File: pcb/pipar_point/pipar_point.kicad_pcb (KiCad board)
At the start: 2 copper layers, 32 parts, among them Y50 Crystal_GND2

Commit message: more pipar poimt progress
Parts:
- added AE1: Antenna, Mikoto:2.4GHz-meander-antenna-v2, B.Cu at (171.4, 61.8)
- added AE1: Antenna, Mikoto-Footprints:2.4GHz-meander-antenna-v2, B.Cu at (-137.7, 167.9)
- added AE2: Antenna, Mikoto:2.4GHz-meander-antenna-v2, B.Cu at (-153.7, 135.4)
- added C1: 4.7uF, Capacitor_SMD:C_0402_1005Metric, B.Cu at (-143.2, 159.1)
- added C1: 4.7uF, Capacitor_SMD:C_0402_1005Metric, B.Cu at (203.4, 69.8)
- added C10: 1.5pF, Capacitor_SMD:C_0402_1005Metric, B.Cu at (-144.8, 169.3)
- added C10: 1.5pF, Capacitor_SMD:C_0402_1005Metric, B.Cu at (198.5, 69.7)
- added C11: 1pF, Capacitor_SMD:C_0402_1005Metric, B.Cu at (196.9, 70.8)
- added C11: 1pF, Capacitor_SMD:C_0402_1005Metric, B.Cu at (-147.8, 168.9)
- added C12: 1pF, Capacitor_SMD:C_0402_1005Metric, B.Cu at (195.3, 71.9)
- added C12: 1pF, Capacitor_SMD:C_0402_1005Metric, B.Cu at (-149.9, 167.6)
- added C13: 4.7uF, Capacitor_SMD:C_0402_1005Metric, B.Cu at (193.7, 73.1)
- added C13: 4.7uF, Capacitor_SMD:C_0402_1005Metric, B.Cu at (-146.0, 157.0)
- added C14: 1uF, Capacitor_SMD:C_0402_1005Metric, B.Cu at (192.1, 74.2)
- added C14: 1uF, Capacitor_SMD:C_0402_1005Metric, B.Cu at (-135.2, 161.8)
- added C15: 1uF, Capacitor_SMD:C_0402_1005Metric, B.Cu at (-133.1, 164.8)
- added C15: 1uF, Capacitor_SMD:C_0402_1005Metric, B.Cu at (200.1, 65.1)
- added C16: 100nF, Capacitor_SMD:C_0402_1005Metric, B.Cu at (198.5, 66.2)
- added C16: 100nF, Capacitor_SMD:C_0402_1005Metric, B.Cu at (-155.1, 156.3)
- added C17: 100nF, Capacitor_SMD:C_0402_1005Metric, B.Cu at (196.9, 67.3)
- added C17: 100nF, Capacitor_SMD:C_0402_1005Metric, B.Cu at (-155.4, 164.1)
- added C18: 100nF, Capacitor_SMD:C_0402_1005Metric, B.Cu at (195.3, 68.4)
- added C18: 100nF, Capacitor_SMD:C_0402_1005Metric, B.Cu at (-141.6, 164.6)
- added C19: 4.7uF, Capacitor_SMD:C_0402_1005Metric, B.Cu at (193.7, 69.6)
- added C19: 4.7uF, Capacitor_SMD:C_0402_1005Metric, B.Cu at (-143.6, 156.5)
- added C2: 1uF, Capacitor_SMD:C_0402_1005Metric, B.Cu at (-151.8, 169.0)
- added C2: 1uF, Capacitor_SMD:C_0402_1005Metric, B.Cu at (201.8, 70.9)
- added C20: 1uF, Capacitor_SMD:C_0402_1005Metric, B.Cu at (192.1, 70.7)
- added C20: 1uF, Capacitor_SMD:C_0402_1005Metric, B.Cu at (-142.0, 162.5)
- added C21: 15pF, Capacitor_SMD:C_0402_1005Metric, B.Cu at (-155.2, 168.9)
- added C21: 15pF, Capacitor_SMD:C_0402_1005Metric, B.Cu at (190.4, 71.8)
- added C22: 15pF, Capacitor_SMD:C_0402_1005Metric, B.Cu at (-155.4, 165.1)
- added C22: 15pF, Capacitor_SMD:C_0402_1005Metric, B.Cu at (198.5, 62.7)
- added C23: 10nF, Capacitor_SMD:C_0402_1005Metric, B.Cu at (-136.2, 164.0)
- added C23: 10nF, Capacitor_SMD:C_0402_1005Metric, B.Cu at (196.9, 63.8)
- added C24: 1000pF/NC, Capacitor_SMD:C_0402_1005Metric, B.Cu at (195.2, 65.0)
- added C25: 1.5pF, Capacitor_SMD:C_0402_1005Metric, B.Cu at (-160.7, 136.8)
- added C26: 1pF, Capacitor_SMD:C_0402_1005Metric, B.Cu at (-164.3, 136.6)
- added C27: 15pF, Capacitor_SMD:C_0402_1005Metric, B.Cu at (-171.5, 137.2)
- added C28: 15pF, Capacitor_SMD:C_0402_1005Metric, B.Cu at (-171.9, 133.1)
- added C29: 1pF, Capacitor_SMD:C_0402_1005Metric, B.Cu at (-166.3, 134.9)
- added C3: 47nF, Capacitor_SMD:C_0402_1005Metric, B.Cu at (-154.2, 159.9)
- added C3: 47nF, Capacitor_SMD:C_0402_1005Metric, B.Cu at (200.2, 72.0)
- added C30: 100nF, Capacitor_SMD:C_0402_1005Metric, B.Cu at (-170.8, 124.3)
- added C31: 100pF, Capacitor_SMD:C_0402_1005Metric, B.Cu at (-169.1, 136.8)
- added C32: 1nF, Capacitor_SMD:C_0402_1005Metric, B.Cu at (-188.6, 182.0)
- added C33: 4.7uF, Capacitor_SMD:C_0402_1005Metric, B.Cu at (-159.5, 125.7)
- added C34: 4.7uF, Capacitor_SMD:C_0402_1005Metric, B.Cu at (-159.5, 126.7)
- added C35: 1uF, Capacitor_SMD:C_0402_1005Metric, B.Cu at (-168.1, 136.8)
- added C36: 47nF, Capacitor_SMD:C_0402_1005Metric, B.Cu at (-171.2, 128.3)
- added C37: 15pF, Capacitor_SMD:C_0402_1005Metric, B.Cu at (-168.8, 124.3)
- added C38: 15pF, Capacitor_SMD:C_0402_1005Metric, B.Cu at (-166.7, 122.9)
- added C39: 4.7uF, Capacitor_SMD:C_0402_1005Metric, B.Cu at (-162.5, 124.2)
- added C4: 4.7uF, Capacitor_SMD:C_0402_1005Metric, B.Cu at (198.6, 73.1)
- added C4: 4.7uF, Capacitor_SMD:C_0402_1005Metric, B.Cu at (-143.2, 158.1)
- added C40: 100nF, Capacitor_SMD:C_0402_1005Metric, B.Cu at (-171.8, 124.3)
- added C41: 10nF, Capacitor_SMD:C_0402_1005Metric, B.Cu at (-192.6, 179.1)
- added C42: 100nF, Capacitor_SMD:C_0402_1005Metric, B.Cu at (-158.4, 132.5)
- added C43: 100nF, Capacitor_SMD:C_0402_1005Metric, B.Cu at (-171.9, 132.1)
- added C44: 4.7uF, Capacitor_SMD:C_0402_1005Metric, B.Cu at (-160.3, 123.8)
- added C45: 1uF, Capacitor_SMD:C_0402_1005Metric, B.Cu at (-158.4, 130.1)
- added C46: 1000pF/NC, Capacitor_SMD:C_0402_1005Metric, B.Cu at (-188.6, 176.2)
- added C47: 1uF, Capacitor_SMD:C_0402_1005Metric, B.Cu at (-190.6, 176.2)
- added C48: 1uF, Capacitor_SMD:C_0402_1005Metric, B.Cu at (-192.6, 176.2)
- added C49: 10uF, Capacitor_SMD:C_0603_1608Metric, B.Cu at (191.6, 77.4)
- added C5: 1nF, Capacitor_SMD:C_0402_1005Metric, B.Cu at (-142.8, 166.5)
- added C5: 1nF, Capacitor_SMD:C_0402_1005Metric, B.Cu at (197.0, 74.3)
- added C6: 100pF, Capacitor_SMD:C_0402_1005Metric, B.Cu at (195.3, 75.4)
- added C6: 100pF, Capacitor_SMD:C_0402_1005Metric, B.Cu at (-152.8, 169.0)
- added C62: 4.7uF, Capacitor_SMD:C_0402_1005Metric, B.Cu at (193.6, 66.1)
- added C63: 10uF, Capacitor_SMD:C_0603_1608Metric, B.Cu at (-197.1, 180.9)
- added C64: 4.7uF, Capacitor_SMD:C_0402_1005Metric, B.Cu at (-194.5, 176.2)
- added C65: 100nF, Capacitor_SMD:C_0402_1005Metric, B.Cu at (192.0, 67.2)
- added C66: 100nF, Capacitor_SMD:C_0402_1005Metric, B.Cu at (-196.5, 176.2)
- added C7: 100nF, Capacitor_SMD:C_0402_1005Metric, B.Cu at (193.7, 76.5)
- added C7: 100nF, Capacitor_SMD:C_0402_1005Metric, B.Cu at (-154.0, 156.3)
- added C8: 15pF, Capacitor_SMD:C_0402_1005Metric, B.Cu at (201.8, 67.4)
- added C8: 15pF, Capacitor_SMD:C_0402_1005Metric, B.Cu at (-152.1, 156.8)
- added C9: 15pF, Capacitor_SMD:C_0402_1005Metric, B.Cu at (200.2, 68.5)
- added C9: 15pF, Capacitor_SMD:C_0402_1005Metric, B.Cu at (-150.1, 155.3)
- added D1: CHG, LED_SMD:LED_0603_1608Metric, B.Cu at (181.8, 79.3)
- added D100: D_Small, Diode_SMD:D_0402_1005Metric, B.Cu at (142.7, 121.5)
- added D101: D_Small, Diode_SMD:D_0402_1005Metric, B.Cu at (152.4, 135.4)
- added D102: D_Small, Diode_SMD:D_0402_1005Metric, B.Cu at (114.0, 114.5)
- added D103: D_Small, Diode_SMD:D_0402_1005Metric, B.Cu at (122.5, 129.2)
- added D104: D_Small, Diode_SMD:D_0402_1005Metric, B.Cu at (130.9, 143.9)
- added D105: D_Small, Diode_SMD:D_0402_1005Metric, B.Cu at (90.6, 111.2)
- added D106: D_Small, Diode_SMD:D_0402_1005Metric, B.Cu at (93.5, 127.9)
- added D107: D_Small, Diode_SMD:D_0402_1005Metric, B.Cu at (96.5, 144.6)
- added D108: D_Small, Diode_SMD:D_0402_1005Metric, B.Cu at (73.4, 118.9)
- added D109: D_Small, Diode_SMD:D_0402_1005Metric, B.Cu at (76.3, 135.6)
- added D110: D_Small, Diode_SMD:D_0402_1005Metric, B.Cu at (-138.0, 132.0)
- added D111: D_Small, Diode_SMD:D_0402_1005Metric, B.Cu at (-123.3, 142.3)
- added D112: D_Small, Diode_SMD:D_0402_1005Metric, B.Cu at (-108.6, 152.6)
- added D113: D_Small, Diode_SMD:D_0402_1005Metric, B.Cu at (-131.4, 76.9)
- added D114: D_Small, Diode_SMD:D_0402_1005Metric, B.Cu at (-132.9, 93.8)
- added D115: D_Small, Diode_SMD:D_0402_1005Metric, B.Cu at (-134.4, 110.7)
- added D116: D_Small, Diode_SMD:D_0402_1005Metric, B.Cu at (-150.1, 71.8)
- added D117: D_Small, Diode_SMD:D_0402_1005Metric, B.Cu at (-151.6, 88.7)
- added D118: D_Small, Diode_SMD:D_0402_1005Metric, B.Cu at (-153.1, 105.6)
- added D119: D_Small, Diode_SMD:D_0402_1005Metric, B.Cu at (-172.8, 70.0)
- added D120: D_Small, Diode_SMD:D_0402_1005Metric, B.Cu at (-172.8, 87.0)
- added D121: D_Small, Diode_SMD:D_0402_1005Metric, B.Cu at (-172.8, 104.0)
- added D122: D_Small, Diode_SMD:D_0402_1005Metric, B.Cu at (-195.2, 76.8)
- added D123: D_Small, Diode_SMD:D_0402_1005Metric, B.Cu at (-193.8, 93.7)
- added D124: D_Small, Diode_SMD:D_0402_1005Metric, B.Cu at (-192.3, 110.6)
- added D125: D_Small, Diode_SMD:D_0402_1005Metric, B.Cu at (-222.4, 101.6)
- added D126: D_Small, Diode_SMD:D_0402_1005Metric, B.Cu at (-215.2, 117.0)
- added D127: D_Small, Diode_SMD:D_0402_1005Metric, B.Cu at (-208.0, 132.3)
- added D128: D_Small, Diode_SMD:D_0402_1005Metric, B.Cu at (-233.8, 120.5)
- added D129: D_Small, Diode_SMD:D_0402_1005Metric, B.Cu at (-226.6, 135.9)
- added D2: B5819W SL, Diode_SMD:D_SOD-323, B.Cu at (186.0, 45.7)
- added D2: B5819W SL, Diode_SMD:D_SOD-323, B.Cu at (-130.2, 159.1)
- added D22: BLUE, LED_SMD:LED_0603_1608Metric, B.Cu at (177.5, 82.3)
- added D23: BLUE, LED_SMD:LED_0603_1608Metric, B.Cu at (-211.4, 176.8)
- added D3: BLUE, LED_SMD:LED_0603_1608Metric, B.Cu at (179.6, 80.8)
- added D4: BLUE, LED_SMD:LED_0603_1608Metric, B.Cu at (-206.3, 176.8)
- added D5: B5819W SL, Diode_SMD:D_SOD-323, B.Cu at (-186.4, 163.6)
- added D6: CHG, LED_SMD:LED_0603_1608Metric, B.Cu at (-208.8, 176.8)
- added D90: D_Small, Diode_SMD:D_0402_1005Metric, B.Cu at (149.7, 24.9)
- added D91: D_Small, Diode_SMD:D_0402_1005Metric, B.Cu at (143.6, 41.7)
- added D92: D_Small, Diode_SMD:D_0402_1005Metric, B.Cu at (137.5, 58.6)
- added D93: D_Small, Diode_SMD:D_0402_1005Metric, B.Cu at (181.5, 104.8)
- added D94: D_Small, Diode_SMD:D_0402_1005Metric, B.Cu at (170.6, 91.8)
- added D95: D_Small, Diode_SMD:D_0402_1005Metric, B.Cu at (159.7, 78.9)
- added D96: D_Small, Diode_SMD:D_0402_1005Metric, B.Cu at (147.3, 93.8)
- added D97: D_Small, Diode_SMD:D_0402_1005Metric, B.Cu at (158.2, 106.7)
- added D98: D_Small, Diode_SMD:D_0402_1005Metric, B.Cu at (169.1, 119.7)
- added D99: D_Small, Diode_SMD:D_0402_1005Metric, B.Cu at (133.0, 107.6)
- added H100: SwitchHoles, Keyboard:SwitchHoles_Kailh_Choc_V1V2, F.Cu at (135.9, 126.2)
- added H101: SwitchHoles, Keyboard:SwitchHoles_Kailh_Choc_V1V2, F.Cu at (145.6, 140.1)
- added H102: SwitchHoles, Keyboard:SwitchHoles_Kailh_Choc_V1V2, F.Cu at (106.8, 118.7)
- added H103: SwitchHoles, Keyboard:SwitchHoles_Kailh_Choc_V1V2, F.Cu at (115.3, 133.4)
- added H104: SwitchHoles, Keyboard:SwitchHoles_Kailh_Choc_V1V2, F.Cu at (123.8, 148.0)
- added H105: SwitchHoles, Keyboard:SwitchHoles_Kailh_Choc_V1V2, F.Cu at (82.4, 112.6)
- added H106: SwitchHoles, Keyboard:SwitchHoles_Kailh_Choc_V1V2, F.Cu at (85.4, 129.3)
- added H107: SwitchHoles, Keyboard:SwitchHoles_Kailh_Choc_V1V2, F.Cu at (88.3, 146.0)
- added H108: SwitchHoles, Keyboard:SwitchHoles_Kailh_Choc_V1V2, F.Cu at (65.2, 120.4)
- added H109: SwitchHoles, Keyboard:SwitchHoles_Kailh_Choc_V1V2, F.Cu at (68.1, 137.1)
- added H110: SwitchHoles, Keyboard:SwitchHoles_Kailh_Choc_V1V2, F.Cu at (-131.2, 136.7)
- added H111: SwitchHoles, Keyboard:SwitchHoles_Kailh_Choc_V1V2, F.Cu at (-116.5, 147.0)
- added H112: SwitchHoles, Keyboard:SwitchHoles_Kailh_Choc_V1V2, F.Cu at (-101.8, 157.3)
- added H113: SwitchHoles, Keyboard:SwitchHoles_Kailh_Choc_V1V2, F.Cu at (-123.1, 77.6)
- added H114: SwitchHoles, Keyboard:SwitchHoles_Kailh_Choc_V1V2, F.Cu at (-124.6, 94.5)
- added H115: SwitchHoles, Keyboard:SwitchHoles_Kailh_Choc_V1V2, F.Cu at (-126.1, 111.4)
- added H116: SwitchHoles, Keyboard:SwitchHoles_Kailh_Choc_V1V2, F.Cu at (-141.9, 72.6)
- added H117: SwitchHoles, Keyboard:SwitchHoles_Kailh_Choc_V1V2, F.Cu at (-143.3, 89.5)
- added H118: SwitchHoles, Keyboard:SwitchHoles_Kailh_Choc_V1V2, F.Cu at (-144.8, 106.3)
- added H119: SwitchHoles, Keyboard:SwitchHoles_Kailh_Choc_V1V2, F.Cu at (-164.5, 70.0)
- added H120: SwitchHoles, Keyboard:SwitchHoles_Kailh_Choc_V1V2, F.Cu at (-164.5, 87.0)
- added H121: SwitchHoles, Keyboard:SwitchHoles_Kailh_Choc_V1V2, F.Cu at (-164.5, 104.0)
- added H122: SwitchHoles, Keyboard:SwitchHoles_Kailh_Choc_V1V2, F.Cu at (-187.0, 76.1)
- added H123: SwitchHoles, Keyboard:SwitchHoles_Kailh_Choc_V1V2, F.Cu at (-185.5, 93.0)
- added H124: SwitchHoles, Keyboard:SwitchHoles_Kailh_Choc_V1V2, F.Cu at (-184.0, 109.9)
- added H125: SwitchHoles, Keyboard:SwitchHoles_Kailh_Choc_V1V2, F.Cu at (-214.8, 98.1)
- added H126: SwitchHoles, Keyboard:SwitchHoles_Kailh_Choc_V1V2, F.Cu at (-207.7, 113.5)
- added H127: SwitchHoles, Keyboard:SwitchHoles_Kailh_Choc_V1V2, F.Cu at (-200.5, 128.8)
- added H128: SwitchHoles, Keyboard:SwitchHoles_Kailh_Choc_V1V2, F.Cu at (-226.3, 117.0)
- added H129: SwitchHoles, Keyboard:SwitchHoles_Kailh_Choc_V1V2, F.Cu at (-219.1, 132.4)
- added H90: SwitchHoles, Keyboard:SwitchHoles_Kailh_Choc_V1V2, F.Cu at (146.9, 32.7)
- added H91: SwitchHoles, Keyboard:SwitchHoles_Kailh_Choc_V1V2, F.Cu at (140.8, 49.5)
- added H92: SwitchHoles, Keyboard:SwitchHoles_Kailh_Choc_V1V2, F.Cu at (134.6, 66.4)
- added H93: SwitchHoles, Keyboard:SwitchHoles_Kailh_Choc_V1V2, F.Cu at (175.2, 110.2)
- added H94: SwitchHoles, Keyboard:SwitchHoles_Kailh_Choc_V1V2, F.Cu at (164.3, 97.2)
- added H95: SwitchHoles, Keyboard:SwitchHoles_Kailh_Choc_V1V2, F.Cu at (153.4, 84.2)
- added H96: SwitchHoles, Keyboard:SwitchHoles_Kailh_Choc_V1V2, F.Cu at (141.0, 99.1)
- added H97: SwitchHoles, Keyboard:SwitchHoles_Kailh_Choc_V1V2, F.Cu at (151.8, 112.1)
- added H98: SwitchHoles, Keyboard:SwitchHoles_Kailh_Choc_V1V2, F.Cu at (162.7, 125.1)
- added H99: SwitchHoles, Keyboard:SwitchHoles_Kailh_Choc_V1V2, F.Cu at (126.2, 112.3)
- added J53: Conn_02x04_Odd_Even, Connector_PinHeader_2.54mm:PinHeader_2x04_P2.54mm_Vertical, F.Cu at (172.2, 46.2)
- added J54: Conn_02x04_Odd_Even, Connector_PinHeader_2.54mm:PinHeader_2x04_P2.54mm_Vertical_SMD, B.Cu at (-228.4, 104.7)
- added KHS100: KHS, Keyboard:Kailh_HS_Socket, F.Cu at (135.2, 120.8)
- added KHS101: KHS, Keyboard:Kailh_HS_Socket, F.Cu at (144.9, 134.7)
- added KHS102: KHS, Keyboard:Kailh_HS_Socket, F.Cu at (106.5, 113.2)
- added KHS103: KHS, Keyboard:Kailh_HS_Socket, F.Cu at (115.0, 127.9)
- added KHS104: KHS, Keyboard:Kailh_HS_Socket, F.Cu at (123.5, 142.5)
- added KHS105: KHS, Keyboard:Kailh_HS_Socket, F.Cu at (84.1, 107.4)
- added KHS106: KHS, Keyboard:Kailh_HS_Socket, F.Cu at (87.0, 124.1)
- added KHS107: KHS, Keyboard:Kailh_HS_Socket, F.Cu at (89.9, 140.8)
- added KHS108: KHS, Keyboard:Kailh_HS_Socket, F.Cu at (66.8, 115.1)
- added KHS109: KHS, Keyboard:Kailh_HS_Socket, F.Cu at (69.8, 131.8)
- added KHS110: KHS, Keyboard:Kailh_HS_Socket, F.Cu at (-136.1, 139.3)
- added KHS111: KHS, Keyboard:Kailh_HS_Socket, F.Cu at (-121.4, 149.6)
- added KHS112: KHS, Keyboard:Kailh_HS_Socket, F.Cu at (-106.7, 159.9)
- added KHS113: KHS, Keyboard:Kailh_HS_Socket, F.Cu at (-126.1, 82.3)
- added KHS114: KHS, Keyboard:Kailh_HS_Socket, F.Cu at (-127.5, 99.2)
- added KHS115: KHS, Keyboard:Kailh_HS_Socket, F.Cu at (-129.0, 116.1)
- added KHS116: KHS, Keyboard:Kailh_HS_Socket, F.Cu at (-144.8, 77.2)
- added KHS117: KHS, Keyboard:Kailh_HS_Socket, F.Cu at (-146.3, 94.1)
- added KHS118: KHS, Keyboard:Kailh_HS_Socket, F.Cu at (-147.7, 111.0)
- added KHS119: KHS, Keyboard:Kailh_HS_Socket, F.Cu at (-167.0, 74.9)
- added KHS120: KHS, Keyboard:Kailh_HS_Socket, F.Cu at (-167.0, 91.9)
- added KHS121: KHS, Keyboard:Kailh_HS_Socket, F.Cu at (-167.0, 108.9)
- added KHS122: KHS, Keyboard:Kailh_HS_Socket, F.Cu at (-189.1, 81.2)
- added KHS123: KHS, Keyboard:Kailh_HS_Socket, F.Cu at (-187.6, 98.1)
- added KHS124: KHS, Keyboard:Kailh_HS_Socket, F.Cu at (-186.1, 115.0)
- added KHS125: KHS, Keyboard:Kailh_HS_Socket, F.Cu at (-215.0, 103.6)
- added KHS126: KHS, Keyboard:Kailh_HS_Socket, F.Cu at (-207.9, 119.0)
- added KHS127: KHS, Keyboard:Kailh_HS_Socket, F.Cu at (-200.7, 134.3)
- added KHS128: KHS, Keyboard:Kailh_HS_Socket, F.Cu at (-226.5, 122.5)
- added KHS129: KHS, Keyboard:Kailh_HS_Socket, F.Cu at (-219.3, 137.9)
- added KHS90: KHS, Keyboard:Kailh_HS_Socket, F.Cu at (143.2, 28.6)
- added KHS91: KHS, Keyboard:Kailh_HS_Socket, F.Cu at (137.0, 45.5)
- added KHS92: KHS, Keyboard:Kailh_HS_Socket, F.Cu at (130.9, 62.4)
- added KHS93: KHS, Keyboard:Kailh_HS_Socket, F.Cu at (174.0, 104.8)
- added KHS94: KHS, Keyboard:Kailh_HS_Socket, F.Cu at (163.0, 91.8)
- added KHS95: KHS, Keyboard:Kailh_HS_Socket, F.Cu at (152.2, 78.8)
- added KHS96: KHS, Keyboard:Kailh_HS_Socket, F.Cu at (139.7, 93.7)
- added KHS97: KHS, Keyboard:Kailh_HS_Socket, F.Cu at (150.6, 106.7)
- added KHS98: KHS, Keyboard:Kailh_HS_Socket, F.Cu at (161.5, 119.7)
- added KHS99: KHS, Keyboard:Kailh_HS_Socket, F.Cu at (125.4, 106.9)
- added L1: 15nH, Inductor_SMD:L_0402_1005Metric, B.Cu at (171.2, 66.9)
- added L1: 15nH, Inductor_SMD:L_0402_1005Metric, B.Cu at (-157.3, 159.9)
- added L2: 10uH, Inductor_SMD:L_0603_1608Metric, B.Cu at (189.5, 78.8)
- added L2: 10uH, Inductor_SMD:L_0603_1608Metric, B.Cu at (-156.7, 158.6)
- added L3: 10uH, Inductor_SMD:L_0603_1608Metric, B.Cu at (-145.7, 155.7)
- added L3: 10uH, Inductor_SMD:L_0603_1608Metric, B.Cu at (187.5, 80.2)
- added L4: 3.9nH, Inductor_SMD:L_0402_1005Metric, B.Cu at (-147.8, 167.9)
- added L4: 3.9nH, Inductor_SMD:L_0402_1005Metric, B.Cu at (169.6, 68.1)
- added L5: 3.9nH, Inductor_SMD:L_0402_1005Metric, B.Cu at (-164.3, 135.6)
- added L6: 15nH, Inductor_SMD:L_0402_1005Metric, B.Cu at (-173.7, 127.8)
- added L7: 10uH, Inductor_SMD:L_0603_1608Metric, B.Cu at (-173.2, 126.5)
- added L8: 10uH, Inductor_SMD:L_0603_1608Metric, B.Cu at (-162.5, 122.9)
- added LED100: LED_Small, LED_SMD:LED_0402_1005Metric, F.Cu at (139.0, 130.5)
- added LED101: LED_Small, LED_SMD:LED_0402_1005Metric, F.Cu at (148.7, 144.4)
- added LED102: LED_Small, LED_SMD:LED_0402_1005Metric, F.Cu at (109.4, 123.2)
- added LED103: LED_Small, LED_SMD:LED_0402_1005Metric, F.Cu at (117.9, 137.9)
- added LED104: LED_Small, LED_SMD:LED_0402_1005Metric, F.Cu at (126.4, 152.6)
- added LED105: LED_Small, LED_SMD:LED_0402_1005Metric, F.Cu at (83.4, 117.8)
- added LED106: LED_Small, LED_SMD:LED_0402_1005Metric, F.Cu at (86.3, 134.5)
- added LED107: LED_Small, LED_SMD:LED_0402_1005Metric, F.Cu at (89.3, 151.2)
- added LED108: LED_Small, LED_SMD:LED_0402_1005Metric, F.Cu at (66.1, 125.5)
- added LED109: LED_Small, LED_SMD:LED_0402_1005Metric, F.Cu at (69.1, 142.3)
- added LED110: LED_Small, LED_SMD:LED_0402_1005Metric, F.Cu at (-128.2, 132.5)
- added LED111: LED_Small, LED_SMD:LED_0402_1005Metric, F.Cu at (-113.5, 142.8)
- added LED112: LED_Small, LED_SMD:LED_0402_1005Metric, F.Cu at (-98.7, 153.1)
- added LED113: LED_Small, LED_SMD:LED_0402_1005Metric, F.Cu at (-122.6, 72.5)
- added LED114: LED_Small, LED_SMD:LED_0402_1005Metric, F.Cu at (-124.1, 89.4)
- added LED115: LED_Small, LED_SMD:LED_0402_1005Metric, F.Cu at (-125.5, 106.3)
- added LED116: LED_Small, LED_SMD:LED_0402_1005Metric, F.Cu at (-141.3, 67.4)
- added LED117: LED_Small, LED_SMD:LED_0402_1005Metric, F.Cu at (-142.8, 84.3)
- added LED118: LED_Small, LED_SMD:LED_0402_1005Metric, F.Cu at (-144.3, 101.2)
- added LED119: LED_Small, LED_SMD:LED_0402_1005Metric, F.Cu at (-164.4, 64.8)
- added LED120: LED_Small, LED_SMD:LED_0402_1005Metric, F.Cu at (-164.4, 81.8)
- added LED121: LED_Small, LED_SMD:LED_0402_1005Metric, F.Cu at (-164.4, 98.7)
- added LED122: LED_Small, LED_SMD:LED_0402_1005Metric, F.Cu at (-187.3, 70.9)
- added LED123: LED_Small, LED_SMD:LED_0402_1005Metric, F.Cu at (-185.9, 87.8)
- added LED124: LED_Small, LED_SMD:LED_0402_1005Metric, F.Cu at (-184.4, 104.7)
- added LED125: LED_Small, LED_SMD:LED_0402_1005Metric, F.Cu at (-217.0, 93.3)
- added LED126: LED_Small, LED_SMD:LED_0402_1005Metric, F.Cu at (-209.8, 108.7)
- added LED127: LED_Small, LED_SMD:LED_0402_1005Metric, F.Cu at (-202.6, 124.1)
- added LED128: LED_Small, LED_SMD:LED_0402_1005Metric, F.Cu at (-228.4, 112.2)
- added LED129: LED_Small, LED_SMD:LED_0402_1005Metric, F.Cu at (-221.2, 127.6)
- added LED90: LED_Small, LED_SMD:LED_0402_1005Metric, F.Cu at (151.8, 34.6)
- added LED91: LED_Small, LED_SMD:LED_0402_1005Metric, F.Cu at (145.7, 51.4)
- added LED92: LED_Small, LED_SMD:LED_0402_1005Metric, F.Cu at (139.5, 68.3)
- added LED93: LED_Small, LED_SMD:LED_0402_1005Metric, F.Cu at (178.5, 114.3)
- added LED94: LED_Small, LED_SMD:LED_0402_1005Metric, F.Cu at (167.6, 101.2)
- added LED95: LED_Small, LED_SMD:LED_0402_1005Metric, F.Cu at (156.8, 88.2)
- added LED96: LED_Small, LED_SMD:LED_0402_1005Metric, F.Cu at (144.4, 103.1)
- added LED97: LED_Small, LED_SMD:LED_0402_1005Metric, F.Cu at (155.1, 116.2)
- added LED98: LED_Small, LED_SMD:LED_0402_1005Metric, F.Cu at (166.1, 129.1)
- added LED99: LED_Small, LED_SMD:LED_0402_1005Metric, F.Cu at (129.2, 116.6)
- added LR100: R_Small, Resistor_SMD:R_0402_1005Metric, F.Cu at (138.4, 129.7)
- added LR101: R_Small, Resistor_SMD:R_0402_1005Metric, F.Cu at (148.1, 143.6)
- added LR102: R_Small, Resistor_SMD:R_0402_1005Metric, F.Cu at (108.9, 122.3)
- added LR103: R_Small, Resistor_SMD:R_0402_1005Metric, F.Cu at (117.4, 137.0)
- added LR104: R_Small, Resistor_SMD:R_0402_1005Metric, F.Cu at (125.9, 151.7)
- added LR105: R_Small, Resistor_SMD:R_0402_1005Metric, F.Cu at (83.2, 116.8)
- added LR106: R_Small, Resistor_SMD:R_0402_1005Metric, F.Cu at (86.1, 133.5)
- added LR107: R_Small, Resistor_SMD:R_0402_1005Metric, F.Cu at (89.1, 150.2)
- added LR108: R_Small, Resistor_SMD:R_0402_1005Metric, F.Cu at (65.9, 124.6)
- added LR109: R_Small, Resistor_SMD:R_0402_1005Metric, F.Cu at (68.9, 141.3)
- added LR110: R_Small, Resistor_SMD:R_0402_1005Metric, F.Cu at (-128.7, 133.3)
- added LR111: R_Small, Resistor_SMD:R_0402_1005Metric, F.Cu at (-114.0, 143.6)
- added LR112: R_Small, Resistor_SMD:R_0402_1005Metric, F.Cu at (-99.3, 153.9)
- added LR113: R_Small, Resistor_SMD:R_0402_1005Metric, F.Cu at (-122.7, 73.5)
- added LR114: R_Small, Resistor_SMD:R_0402_1005Metric, F.Cu at (-124.2, 90.4)
- added LR115: R_Small, Resistor_SMD:R_0402_1005Metric, F.Cu at (-125.6, 107.3)
- added LR116: R_Small, Resistor_SMD:R_0402_1005Metric, F.Cu at (-141.4, 68.4)
- added LR117: R_Small, Resistor_SMD:R_0402_1005Metric, F.Cu at (-142.9, 85.3)
- added LR118: R_Small, Resistor_SMD:R_0402_1005Metric, F.Cu at (-144.4, 102.2)
- added LR119: R_Small, Resistor_SMD:R_0402_1005Metric, F.Cu at (-164.4, 65.8)
- added LR120: R_Small, Resistor_SMD:R_0402_1005Metric, F.Cu at (-164.4, 82.8)
- added LR121: R_Small, Resistor_SMD:R_0402_1005Metric, F.Cu at (-164.4, 99.7)
- added LR122: R_Small, Resistor_SMD:R_0402_1005Metric, F.Cu at (-187.2, 71.9)
- added LR123: R_Small, Resistor_SMD:R_0402_1005Metric, F.Cu at (-185.8, 88.8)
- added LR124: R_Small, Resistor_SMD:R_0402_1005Metric, F.Cu at (-184.3, 105.7)
- added LR125: R_Small, Resistor_SMD:R_0402_1005Metric, F.Cu at (-216.5, 94.2)
- added LR126: R_Small, Resistor_SMD:R_0402_1005Metric, F.Cu at (-209.4, 109.6)
- added LR127: R_Small, Resistor_SMD:R_0402_1005Metric, F.Cu at (-202.2, 125.0)
- added LR128: R_Small, Resistor_SMD:R_0402_1005Metric, F.Cu at (-227.9, 113.1)
- added LR129: R_Small, Resistor_SMD:R_0402_1005Metric, F.Cu at (-220.8, 128.5)
- added LR90: R_Small, Resistor_SMD:R_0402_1005Metric, F.Cu at (150.9, 34.2)
- added LR91: R_Small, Resistor_SMD:R_0402_1005Metric, F.Cu at (144.7, 51.1)
- added LR92: R_Small, Resistor_SMD:R_0402_1005Metric, F.Cu at (138.6, 68.0)
- added LR93: R_Small, Resistor_SMD:R_0402_1005Metric, F.Cu at (177.8, 113.5)
- added LR94: R_Small, Resistor_SMD:R_0402_1005Metric, F.Cu at (167.0, 100.4)
- added LR95: R_Small, Resistor_SMD:R_0402_1005Metric, F.Cu at (156.1, 87.4)
- added LR96: R_Small, Resistor_SMD:R_0402_1005Metric, F.Cu at (143.7, 102.3)
- added LR97: R_Small, Resistor_SMD:R_0402_1005Metric, F.Cu at (154.5, 115.4)
- added LR98: R_Small, Resistor_SMD:R_0402_1005Metric, F.Cu at (165.5, 128.3)
- added LR99: R_Small, Resistor_SMD:R_0402_1005Metric, F.Cu at (128.6, 115.8)
- added NT1: NetTie_2, Mikoto-Footprints:net-tie-2-tiny, B.Cu at (-150.2, 164.8)
- added NT1: NetTie_2, Mikoto:net-tie-2-tiny, B.Cu at (161.5, 61.1)
- added NT2: NetTie_2, Mikoto:net-tie-2-tiny, B.Cu at (-166.5, 132.4)
- added P1: USB-C, Connector_USB:USB_C_Receptacle_HRO_TYPE-C-31-M-12, B.Cu at (190.4, 59.5)
- added P2: USB-C, Connector_USB:USB_C_Receptacle_HRO_TYPE-C-31-M-12, B.Cu at (-121.2, 125.8)
- added Q1: AO3416 N-channel MOSFET, Package_TO_SOT_SMD:SOT-23, B.Cu at (181.8, 49.1)
- added Q2: AO3416 N-channel MOSFET, Package_TO_SOT_SMD:SOT-23, B.Cu at (-191.8, 164.0)
- added R1: 0R, Resistor_SMD:R_0402_1005Metric, B.Cu at (167.9, 69.2)
- added R1: 0R, Resistor_SMD:R_0402_1005Metric, B.Cu at (-144.8, 167.8)
- added R10: 10M, Resistor_SMD:R_0402_1005Metric, B.Cu at (-136.2, 165.0)
- added R10: 10M, Resistor_SMD:R_0402_1005Metric, B.Cu at (167.9, 62.1)
- added R11: 1M, Resistor_SMD:R_0402_1005Metric, B.Cu at (166.2, 63.3)
- added R12: 0R, Resistor_SMD:R_0402_1005Metric, B.Cu at (-160.7, 135.6)
- added R13: 2M, Resistor_SMD:R_0603_1608Metric, B.Cu at (-204.6, 180.9)
- added R14: 2M, Resistor_SMD:R_0603_1608Metric, B.Cu at (-207.2, 180.9)
- added R15: 10M, Resistor_SMD:R_0402_1005Metric, B.Cu at (-216.6, 172.5)
- added R16: 1.5k, Resistor_SMD:R_0402_1005Metric, B.Cu at (-210.6, 169.6)
- added R17: 1M, Resistor_SMD:R_0402_1005Metric, B.Cu at (-212.6, 169.6)
- added R18: 2.7k, Resistor_SMD:R_0603_1608Metric, B.Cu at (-209.7, 180.9)
- added R19: 10k, Resistor_SMD:R_0402_1005Metric, B.Cu at (-214.6, 169.6)
- added R2: 10k, Resistor_SMD:R_0402_1005Metric, B.Cu at (166.3, 70.3)
- added R2: 10k, Resistor_SMD:R_0402_1005Metric, B.Cu at (-134.6, 159.6)
- added R20: 5.1k, Resistor_SMD:R_0402_1005Metric, B.Cu at (-216.6, 169.6)
- added R21: 5.1k, Resistor_SMD:R_0402_1005Metric, B.Cu at (-210.6, 166.7)
- added R22: 10k, Resistor_SMD:R_0402_1005Metric, B.Cu at (-212.6, 166.7)
- added R23: 2M, Resistor_SMD:R_0402_1005Metric, B.Cu at (164.6, 64.4)
- added R24: 2M, Resistor_SMD:R_0402_1005Metric, B.Cu at (-214.6, 166.7)
- added R3: 2.7k, Resistor_SMD:R_0603_1608Metric, B.Cu at (185.4, 81.7)
- added R3: 2.7k, Resistor_SMD:R_0603_1608Metric, B.Cu at (-130.1, 162.6)
- added R31: 1.5k, Resistor_SMD:R_0402_1005Metric, B.Cu at (163.0, 65.6)
- added R32: 1.5k, Resistor_SMD:R_0402_1005Metric, B.Cu at (-216.6, 166.7)
- added R39: 4.7k, Resistor_SMD:R_0402_1005Metric_Pad0.72x0.64mm_HandSolder, B.Cu at (163.8, 61.3)
- added R4: 10k, Resistor_SMD:R_0402_1005Metric, B.Cu at (169.5, 64.5)
- added R4: 10k, Resistor_SMD:R_0402_1005Metric, B.Cu at (-135.2, 162.9)
- added R40: 4.7k, Resistor_SMD:R_0402_1005Metric_Pad0.72x0.64mm_HandSolder, B.Cu at (-213.5, 163.6)
- added R5: 1.5k, Resistor_SMD:R_0402_1005Metric, B.Cu at (167.9, 65.7)
- added R6: 5.1k, Resistor_SMD:R_0402_1005Metric, B.Cu at (166.3, 66.8)
- added R7: 5.1k, Resistor_SMD:R_0402_1005Metric, B.Cu at (164.6, 68.0)
- added R8: 2M, Resistor_SMD:R_0603_1608Metric, B.Cu at (183.3, 83.1)
- added R8: 2M, Resistor_SMD:R_0603_1608Metric, B.Cu at (-135.9, 159.7)
- added R9: 2M, Resistor_SMD:R_0603_1608Metric, B.Cu at (181.3, 84.6)
- added R9: 2M, Resistor_SMD:R_0603_1608Metric, B.Cu at (-137.5, 161.0)
- added SW1: Reset, Keyboard:SW4-SMD-2.8-2.6X1.6X0.53MM, B.Cu at (174.7, 72.4)
- added SW2: Reset, Keyboard:SW4-SMD-2.8-2.6X1.6X0.53MM, B.Cu at (-208.1, 167.2)
- added TP5: VBAT, TestPoint:TestPoint_Pad_2.5x2.5mm, B.Cu at (188.3, 74.4)
- added TP6: BAT GND, TestPoint:TestPoint_Pad_2.5x2.5mm, B.Cu at (184.6, 77.0)
- added TP7: VBAT, TestPoint:TestPoint_Pad_2.5x2.5mm, B.Cu at (-197.9, 166.9)
- added TP8: BAT GND, TestPoint:TestPoint_Pad_2.5x2.5mm, B.Cu at (-202.4, 166.9)
- added U1: BQ21040DBVR, BQ21040:SOT95P280X145-6N, B.Cu at (-132.5, 161.7)
- added U1: BQ21040DBVR, Mikoto:SOT95P280X145-6N, B.Cu at (188.1, 50.0)
- added U10: MAX17048, Package_DFN_QFN:TDFN-8-1EP_2x2mm_P0.5mm_EP0.8x1.2mm, B.Cu at (-216.2, 180.2)
- added U2: nRF52840, Package_DFN_QFN:Nordic_AQFN-73-1EP_7x7mm_P0.5mm, B.Cu at (-148.7, 162.3)
- added U2: nRF52840, Package_DFN_QFN:Nordic_AQFN-73-1EP_7x7mm_P0.5mm, B.Cu at (177.5, 58.1)
- added U3: ESDR0502NMUTAG, Mikoto:UDFN-6_1.2x1.0mm_P0.4mm, B.Cu at (162.3, 62.9)
- added U4: nRF52840, Package_DFN_QFN:Nordic_AQFN-73-1EP_7x7mm_P0.5mm, B.Cu at (-165.0, 129.8)
- added U5: ESDR0502NMUTAG, Mikoto:UDFN-6_1.2x1.0mm_P0.4mm, B.Cu at (-215.7, 164.1)
- added U6: BQ21040DBVR, Mikoto:SOT95P280X145-6N, B.Cu at (-187.1, 168.4)
- added U7: XC6220B331MR, Package_TO_SOT_SMD:SOT-23-5, B.Cu at (184.7, 53.2)
- added U8: XC6220B331MR, Package_TO_SOT_SMD:SOT-23-5, B.Cu at (-191.8, 169.0)
- added U9: MAX17048, Package_DFN_QFN:TDFN-8-1EP_2x2mm_P0.5mm_EP0.8x1.2mm, B.Cu at (171.5, 76.9)
- added Y1: 32.768 kHz, Crystal:Crystal_SMD_2012-2Pin_2.0x1.2mm, B.Cu at (-150.2, 156.8)
- added Y1: 32.768 kHz, Crystal:Crystal_SMD_2012-2Pin_2.0x1.2mm, B.Cu at (165.6, 59.7)
- added Y2: 32MHz, Crystal:Crystal_SMD_2016-4Pin_2.0x1.6mm, B.Cu at (-155.0, 167.0)
- added Y2: 32MHz, Crystal:Crystal_SMD_2016-4Pin_2.0x1.6mm, B.Cu at (169.2, 73.6)
- added Y3: 32MHz, Crystal:Crystal_SMD_2016-4Pin_2.0x1.6mm, B.Cu at (-171.5, 135.4)
- added Y4: 32.768 kHz, Crystal:Crystal_SMD_2012-2Pin_2.0x1.2mm, B.Cu at (-166.9, 124.3)
- C50, C51, C52, C53, C54, C55, C56, C57, C58, C59, C60, C61, R50, R51, R52, R53, R54, R55, R56, R57, R58, R59, R60, R61, R62, R63, R64, R65, U50, U51, Y50: moved to B.Cu
- moved C50 65.6 mm to (212.7, 111.3), turned to 125 degrees
- moved C51 64.0 mm to (213.2, 108.5), turned to -145 degrees
- moved C52 60.4 mm to (212.1, 106.7), turned to -55 degrees
- moved R50 58.5 mm to (210.8, 107.1), turned to 125 degrees
- moved R51 57.5 mm to (209.9, 107.7), turned to 125 degrees
- moved R52 56.4 mm to (210.7, 105.0), turned to 35 degrees
- moved R55 54.5 mm to (210.1, 104.1), turned to 35 degrees
- moved U50 54.2 mm to (206.3, 111.0), turned to -145 degrees
- moved R54 53.7 mm to (208.9, 105.5), turned to -55 degrees
- moved R56 52.7 mm to (209.5, 103.2), turned to 35 degrees
- moved C55 50.9 mm to (208.9, 102.3), turned to -145 degrees
- moved R57 50.4 mm to (207.8, 103.9), turned to -55 degrees
- moved C59 48.2 mm to (208.2, 100.7), turned to 125 degrees
- moved C60 47.1 mm to (207.1, 101.4), turned to 125 degrees
- moved C53 40.4 mm to (200.6, 106.4), turned to 125 degrees
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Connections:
- R60 pad 1: /Trackpointer/Vcc -> /Keymatrix/Vcc
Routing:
- net /Keymatrix_left/Vcc: track 0.00 -> 562.7 mm
- net /Keymatrix_left/LEDOut: track 0.00 -> 407.4 mm, vias 0 -> 24
- net /Keymatrix_left/Row1: track 0.00 -> 186.7 mm, vias 0 -> 10
- net /Keymatrix_left/Row2: track 0.00 -> 179.2 mm, vias 0 -> 10
- net /Keymatrix_left/Row0: track 0.00 -> 174.5 mm, vias 0 -> 4
- net /Keymatrix_left/Col0: track 0.00 -> 39.0 mm
- net /Keymatrix_left/Col4: track 0.00 -> 34.9 mm
- net /Keymatrix_left/Col3: track 0.00 -> 34.9 mm
- net /Keymatrix_left/Col5: track 0.00 -> 34.9 mm
- net /Keymatrix_left/Col2: track 0.00 -> 34.9 mm
- net /Keymatrix_left/Col1: track 0.00 -> 34.4 mm
- net /Keymatrix_left/Col6: track 0.00 -> 17.4 mm
- net /Trackpointer/TP_D: track 25.7 -> 32.1 mm, vias 3 -> 4
- net Net-(D117-A): track 0.00 -> 3.31 mm
- net Net-(D120-A): track 0.00 -> 3.31 mm
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
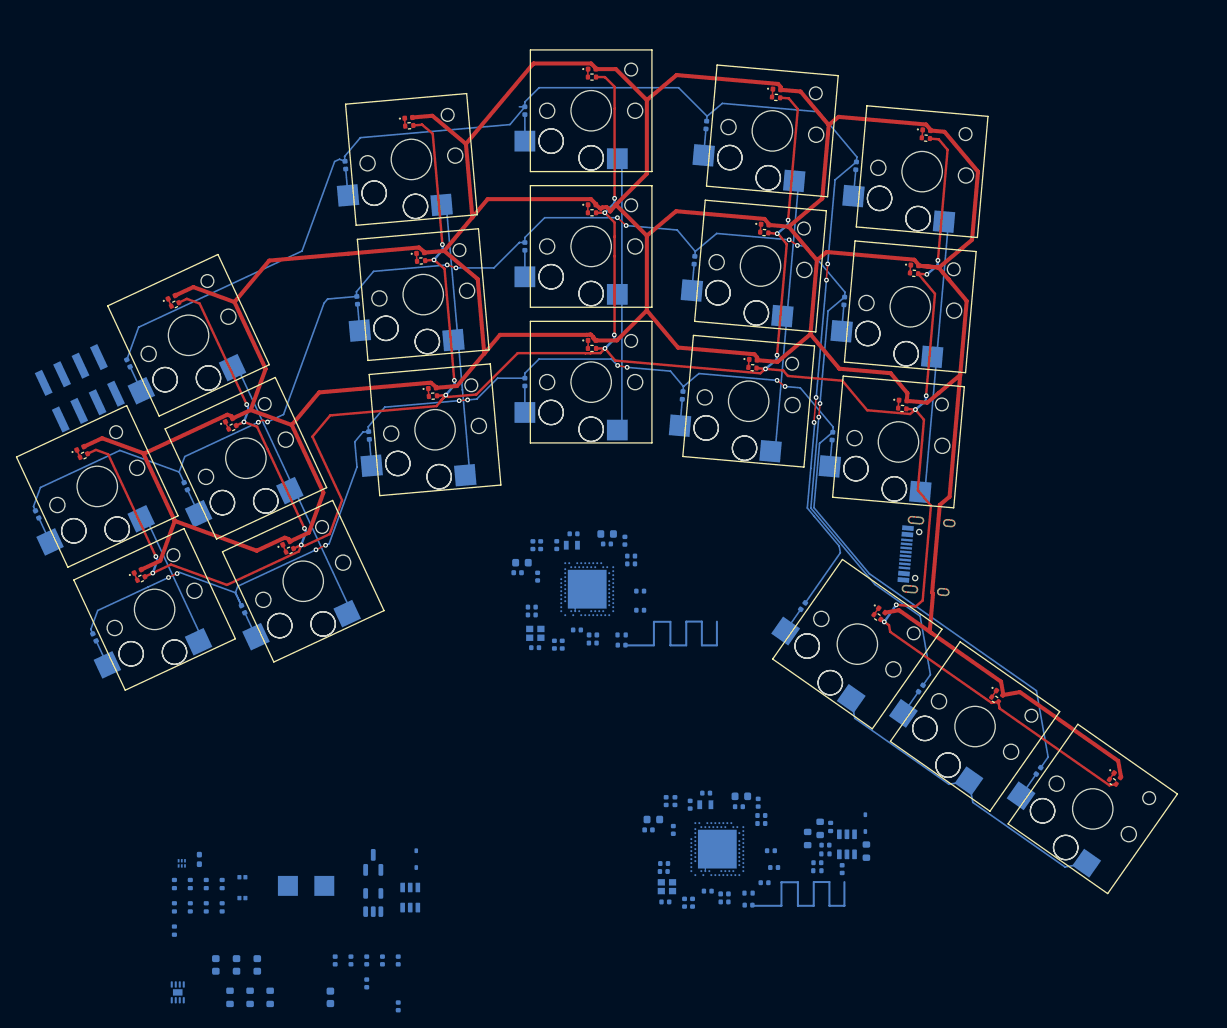
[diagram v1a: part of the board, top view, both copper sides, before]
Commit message: more progress on pipar point
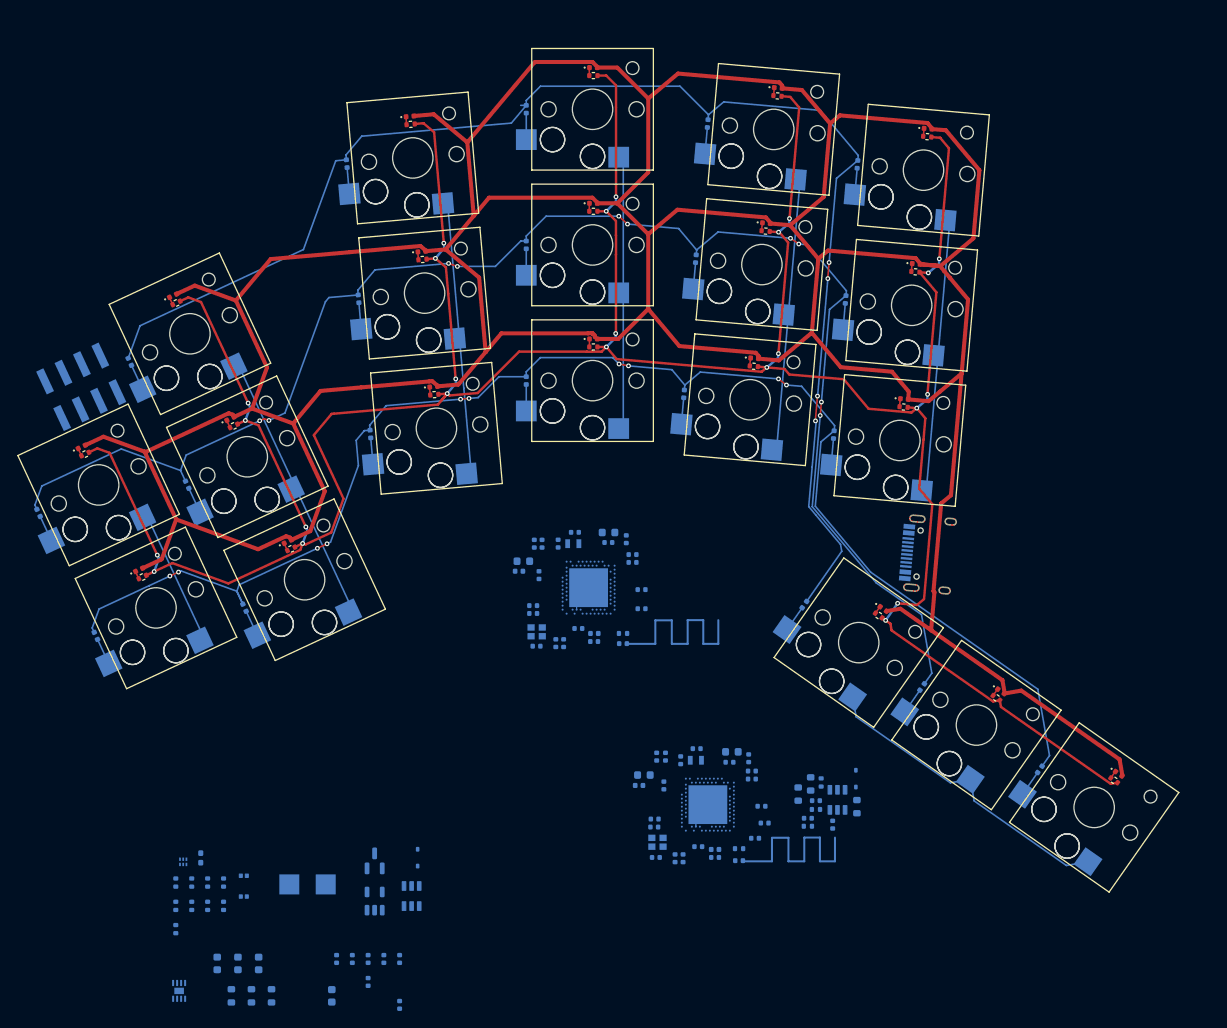
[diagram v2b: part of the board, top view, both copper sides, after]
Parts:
- moved C16 5.68 mm to (-156.3, 150.8)
- moved U2 5.68 mm to (-149.9, 156.8)
- moved C10 5.68 mm to (-146.0, 163.8)
- moved C9 5.68 mm to (-151.3, 149.8)
- moved R4 5.68 mm to (-136.4, 157.4)
- moved C19 5.68 mm to (-144.8, 151.0)
- moved C2 5.68 mm to (-153.0, 163.5)
- moved C3 5.68 mm to (-155.4, 154.4)
- moved C6 5.68 mm to (-154.0, 163.5)
- moved NT1 5.68 mm to (-151.4, 159.3)
- moved R8 5.68 mm to (-137.1, 154.2)
- moved C12 5.68 mm to (-151.1, 162.0)
- moved C7 5.68 mm to (-155.2, 150.8)
- moved C13 5.68 mm to (-147.2, 151.5)
- moved C20 5.68 mm to (-143.2, 157.0)
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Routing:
- net /Keymatrix_left/Vcc: track 562.7 -> 561.7 mm
